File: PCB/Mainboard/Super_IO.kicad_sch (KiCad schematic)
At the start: 24 parts, among them U22 FDC37C665IR, U23 EA, U25 E4

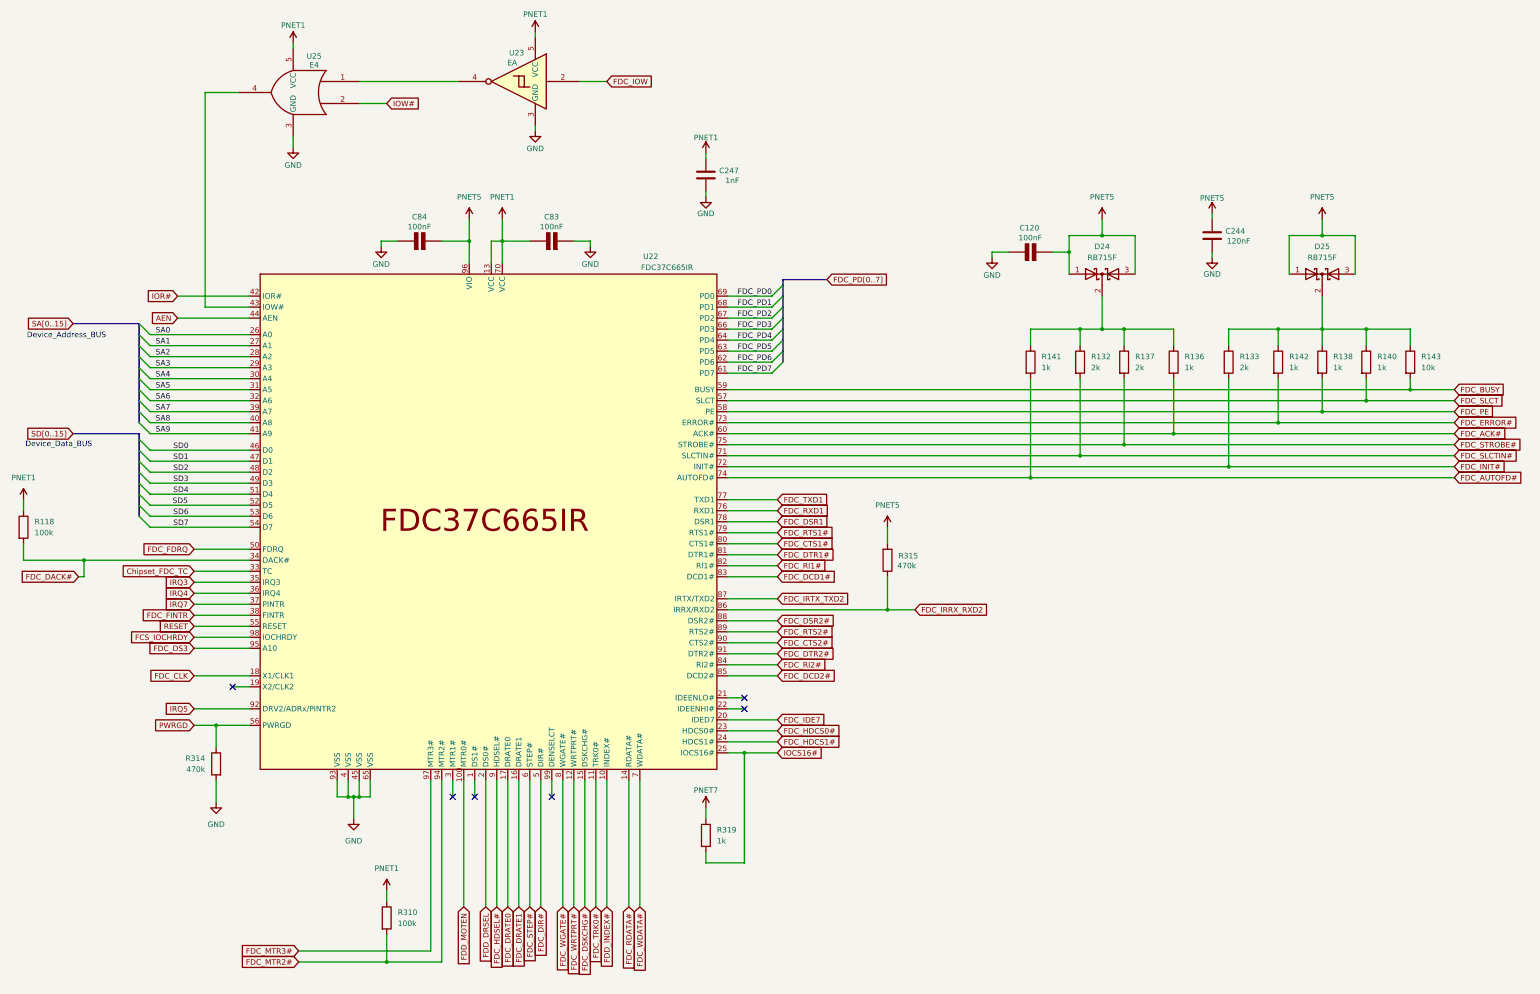
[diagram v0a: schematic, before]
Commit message: Add files via upload
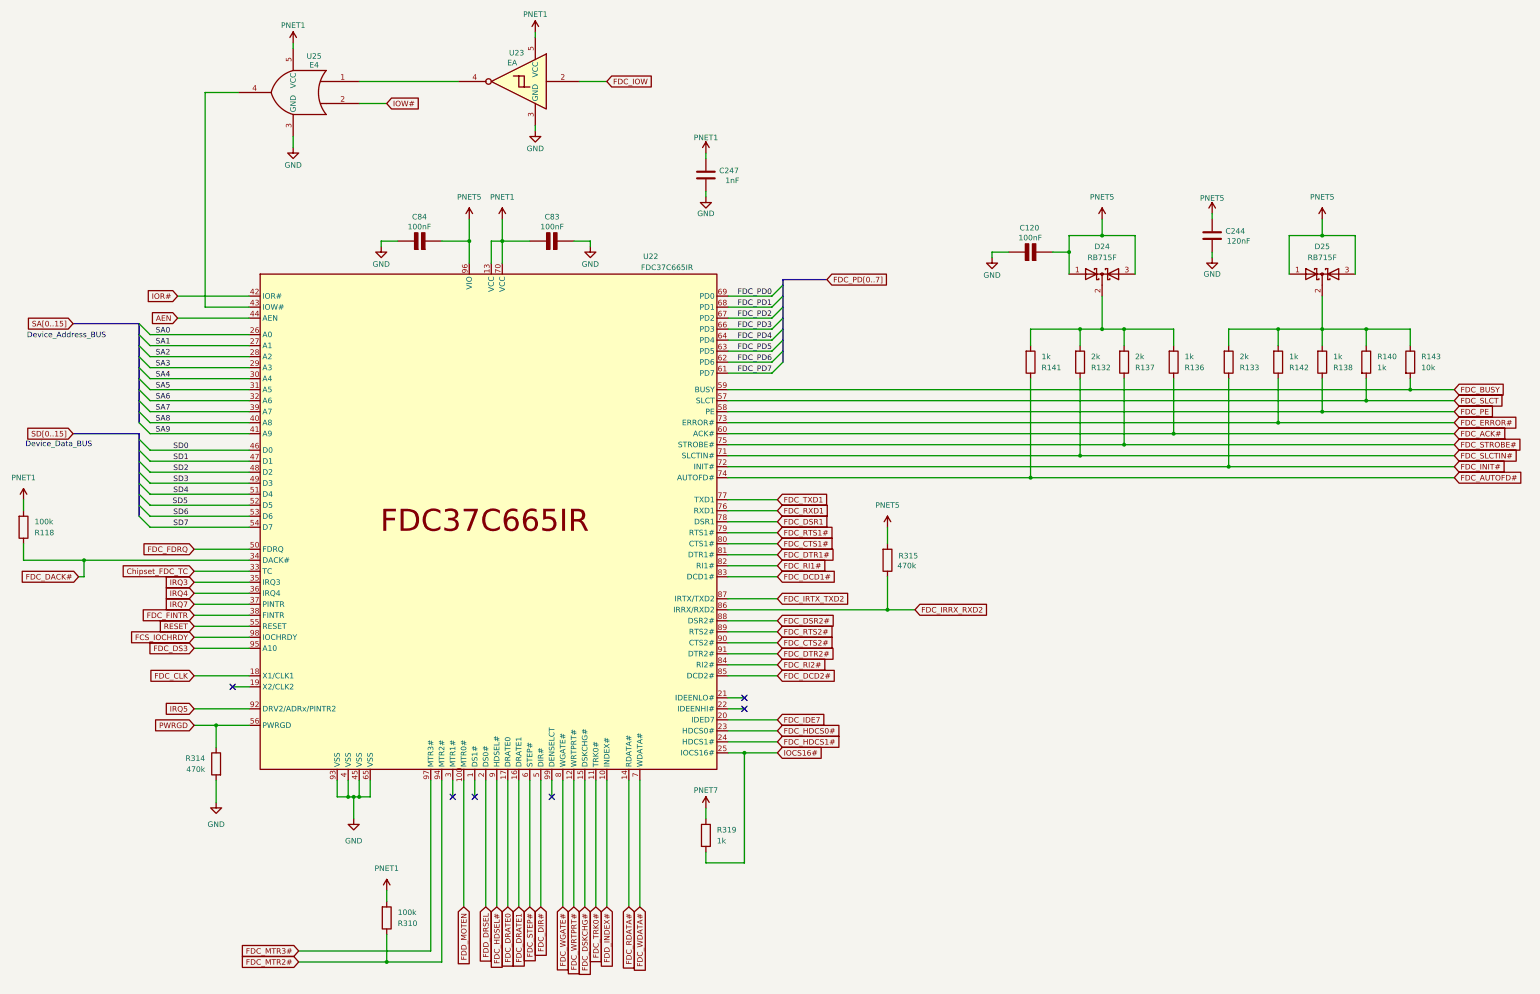
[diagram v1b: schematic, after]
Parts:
- C120, C244, C247, C83, C84: footprint (none) -> Capacitor_SMD:C_0402_1005Metric
- D24, D25: footprint (none) -> PC110:3D
- R118, R132, R133, R136, R137, R138, R140, R141, R142, R143, R314, R319: footprint (none) -> PCM_Resistor_SMD_AKL:R_0402_1005Metric
- R310, R315: footprint (none) -> Resistor_SMD:R_0402_1005Metric
- U22: footprint (none) -> PC110:FDC
- U23, U25: footprint (none) -> PC110:SOT-353
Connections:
- net FDC_ACK#: now also R136.1; no longer R136.2
- net FDC_AUTOFD#: now also R141.1; no longer R141.2
- net FDC_DACK#: now also R118.1; no longer R118.2
- net FDC_ERROR#: now also R142.1; no longer R142.2
- net FDC_INIT#: now also R133.1; no longer R133.2
- net FDC_MTR2#: now also R310.1; no longer R310.2
- net FDC_PE: now also R138.1; no longer R138.2
- net FDC_SLCTIN#: now also R132.1; no longer R132.2
- net FDC_STROBE#: now also R137.1; no longer R137.2
- net GND: now also C83.2 (-); no longer C83.1 (+)
- net PNET1: now also C83.1 (+), R118.2, R310.2; no longer C83.2 (-), R118.1, R310.1
- net at D25.2 (K), R140.1, R143.1: now also R133.2, R138.2, R142.2; no longer R133.1, R138.1, R142.1
- new net: D24.2 (K), R132.2, R136.2, R137.2, R141.2
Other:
- moved on the sheet: C83
